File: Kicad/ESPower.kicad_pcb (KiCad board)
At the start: 2 copper layers, 84.6 x 14.5 mm, 35 parts, among them Q1 DMP2035U-7, Q2 FS8205A, SW2 A, SW3 B, U1 TP4056, U2 DW01A, U3 SPX3819M5-L-3-3, U4 TPS3839DBZ

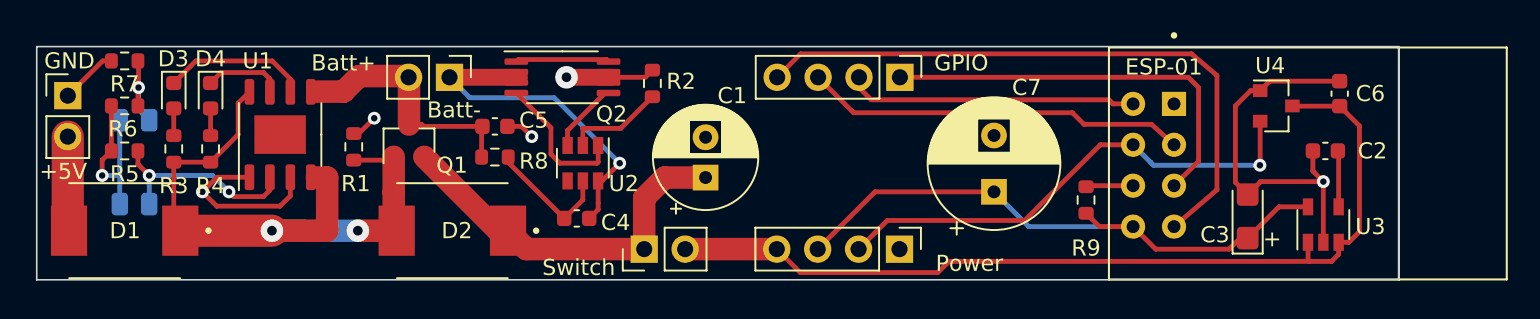
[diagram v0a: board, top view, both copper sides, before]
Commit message: Final routing
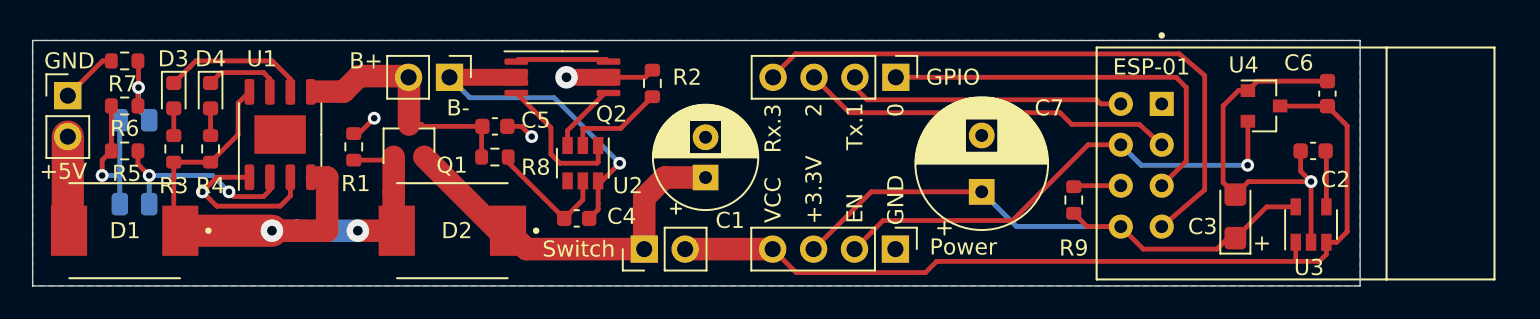
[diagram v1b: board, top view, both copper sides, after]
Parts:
- moved C2 0.76 mm to (157.0, 100.7)
- moved C3 0.76 mm to (152.1, 104.8)
- moved C6 0.76 mm to (157.9, 97.2)
- moved C7 0.76 mm to (136.4, 103.3)
- moved ESP-01 0.76 mm to (155.9, 101.6)
- moved R9 0.76 mm to (142.1, 103.8)
- moved U3 0.76 mm to (156.8, 105.3)
- moved U4 0.76 mm to (153.9, 97.9)
- moved GPIO 0.25 mm to (131.1, 96.1)
- moved Power 0.25 mm to (131.0, 106.8)
- renumbered SW2 to A, SW3 to B, Batt+ to B+
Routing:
- net VDD: track 56.8 -> 55.7 mm
- net +3V3: track 37.8 -> 37.3 mm
- net Net-(J3-Pad2): track 31.0 -> 30.5 mm
- net Net-(J5-Pad2): track 18.1 -> 17.6 mm
- net Net-(J5-Pad3): track 23.8 -> 23.3 mm
- net Net-(J5-Pad1): track 25.5 -> 25.0 mm
- added copper zone on B.Cu, net GND
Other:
- board size 84.6 x 14.5 mm -> 82.4 x 15.2 mm
- board text added: "(cc) BY-NC-SA - 2022 www.agius-industries.eu"
- board text added: "+3.3V"
- board text added: "0"
- board text added: "0 0 250mA 0 1 330mA 1 0 500mA 1 1 1A"
- board text added: "0: VCC=Batt 1: VCC=Input|Batt"
- board text added: "2"
- board text added: "A B Current"
- board text added: "B-"
- board text added: "EN"
- board text added: "ESPower v1.0"
- board text added: "GND"
- board text added: "Rx.3"
- board text added: "Tx.1"
- board text added: "VCC"
- board text removed: "Batt-"
- board text removed: "TODO: Power path select On : Enable powerpath, Input 5V only off : Only battery, Input 5-8v (solar panel)"
